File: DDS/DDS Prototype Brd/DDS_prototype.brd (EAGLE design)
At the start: 36.3 x 12.7 mm, 31 parts, among them T1 ADTT1-6+, U1 AD9913, U2 S-1711A1818-I6T1U, Y1 TSX-3225 25.0000MF10P-C0

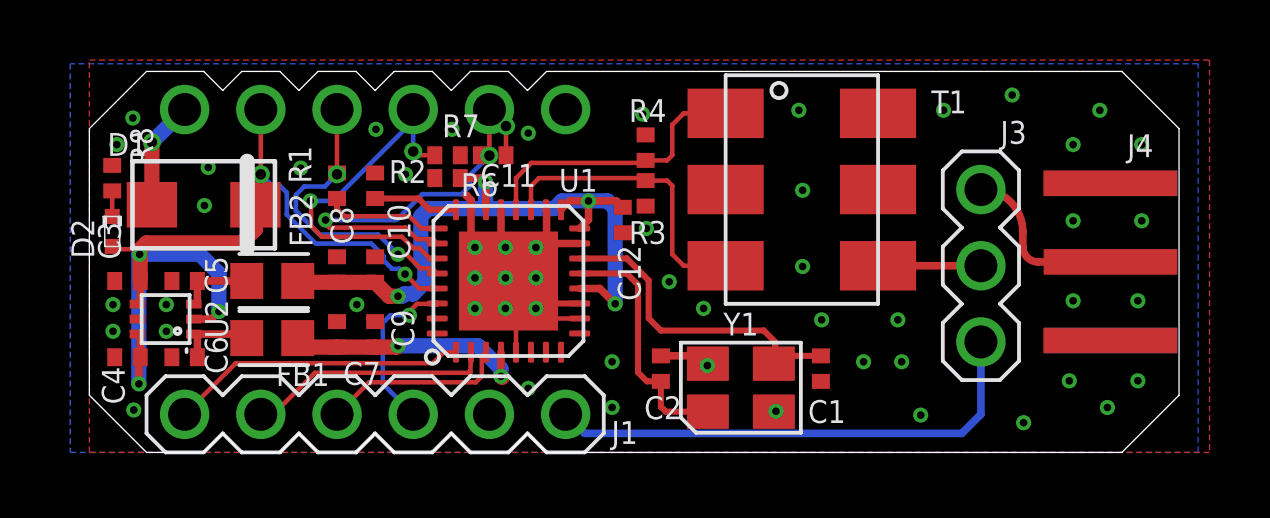
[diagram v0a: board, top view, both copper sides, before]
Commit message: final edits to prototype board. added bom.
final edits to prototype board. added bom. made 3d packages.
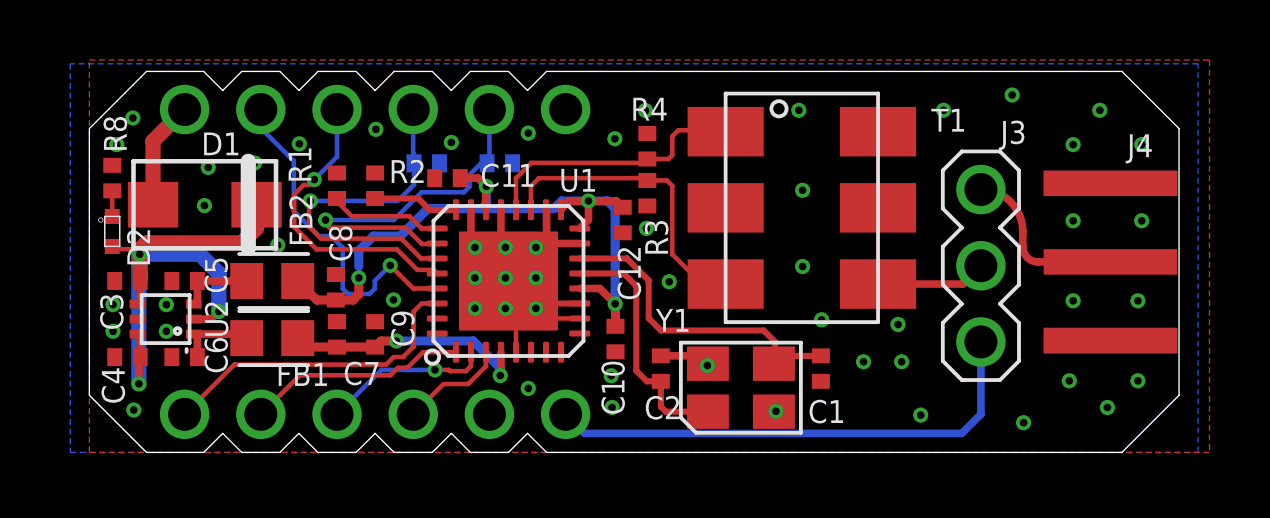
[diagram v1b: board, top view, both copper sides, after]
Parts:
- R1: value (none) -> 100k
- R2: value (none) -> 4.65k
- moved C10 8.34 mm to (17.5, 3.78), turned to 90 degrees
- moved R6 0.74 mm to (11.2, 9.64), flipped to the bottom, turned to 0 degrees
- moved T1 0.61 mm to (23.7, 8.15)
- moved C8 0.59 mm to (8.22, 5.51)
- moved R7 0.34 mm to (13.7, 9.64), flipped to the bottom
- moved R4 0.07 mm to (18.6, 10.2)
- moved R3 0.06 mm to (18.6, 8.64)
- flipped J1 to the bottom, turned to 0 degrees
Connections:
- net PS0: now also J1.P$4; no longer J1.P$3
- net PS1: now also J1.P$3; no longer J1.P$2
- net PS2: now also J1.P$2; no longer J1.P$1
- net SCLK: now also J1.P$1; no longer J1.P$4
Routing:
- net SCLK: track 5.65 -> 10.6 mm, vias 1 -> 0
- net PS0: track 6.21 -> 3.56 mm
- net PS1: track 8.24 -> 5.63 mm, vias 0 -> 1
- net PS2: track 9.90 -> 7.36 mm
- net PWR_DWN_CTRL: track 14.0 -> 12.4 mm, vias 3 -> 1
- net SDIO: track 10.1 -> 11.4 mm, vias 2 -> 1
- net IO_UPDATE: track 12.6 -> 11.8 mm, vias 3 -> 1
- net GND: track 18.1 -> 17.6 mm, vias 54 -> 55
- net CS_N: track 9.92 -> 10.0 mm, vias 2 -> 1
- net 3V3: track 3.63 -> 3.61 mm, vias 1 -> 0
